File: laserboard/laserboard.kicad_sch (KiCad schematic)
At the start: 32 parts, among them U1 AD8656 (1/2 equivalent), U2 AD8656 (1/2 equivalent), U3 AD8656 (1/2 equivalent), U4 AD8656 (1/2 equivalent)

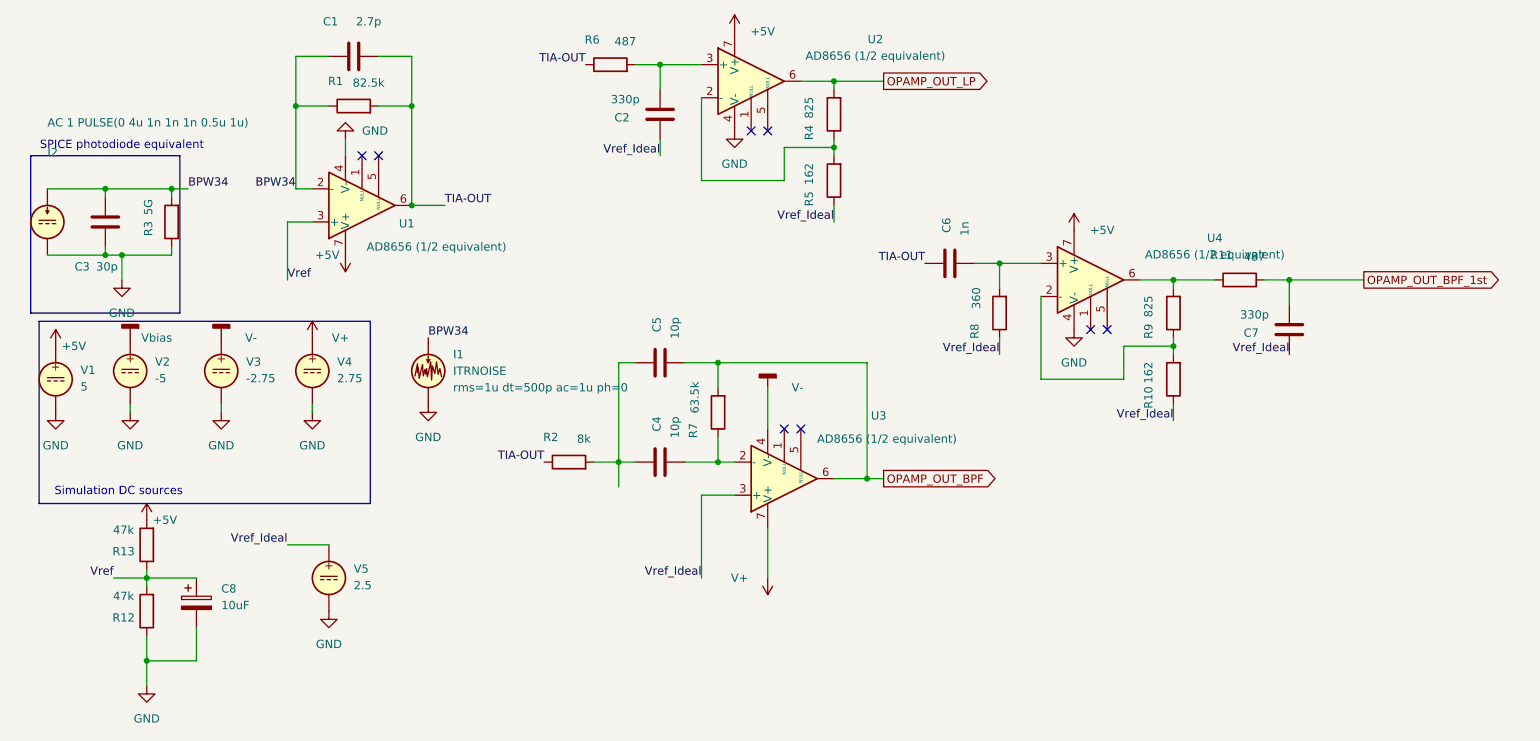
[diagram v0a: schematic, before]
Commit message: Backup
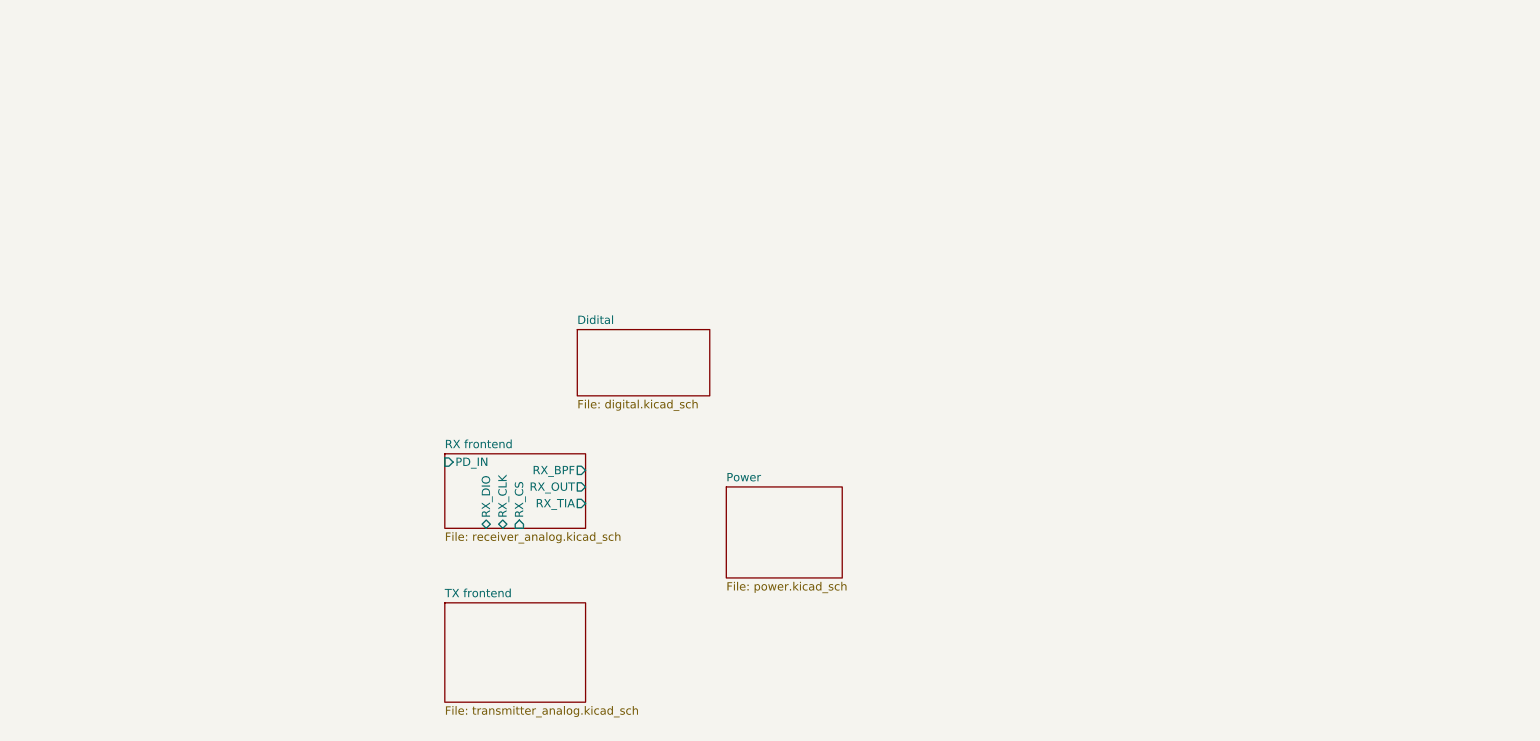
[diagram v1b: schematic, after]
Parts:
- removed C1: 2.7p, symbol Device:C
- removed C2, C7: 330p, symbol Device:C
- removed C3: 30p, symbol Device:C
- removed C4, C5: 10p, symbol Device:C
- removed C6: 1n, symbol Device:C
- removed C8: 10uF, symbol Device:C_Polarized
- removed I1: ITRNOISE, symbol Simulation_SPICE:ITRNOISE
- removed I2: AC 1 PULSE(0 4u 1n 1n 1n 0.5u 1u), symbol Simulation_SPICE:IDC
- removed R1: 82.5k, symbol Device:R
- removed R10, R5: 162, symbol Device:R
- removed R11, R6: 487, symbol Device:R
- removed R12, R13: 47k, symbol Device:R
- removed R2: 8k, symbol Device:R
- removed R3: 5G, symbol Device:R
- removed R4, R9: 825, symbol Device:R
- removed R7: 63.5k, symbol Device:R
- removed R8: 360, symbol Device:R
- removed U1, U2, U3, U4: AD8656 (1/2 equivalent), symbol Amplifier_Operational:AD8655
- removed V1: 5, symbol Simulation_SPICE:VDC
- removed V2: -5, symbol Simulation_SPICE:VDC
- removed V3: -2.75, symbol Simulation_SPICE:VDC
- removed V4: 2.75, symbol Simulation_SPICE:VDC
- removed V5: 2.5, symbol Simulation_SPICE:VDC
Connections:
- no-connect marks 8 -> 0
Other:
- added sheet Didital (digital.kicad_sch)
- added sheet Power (power.kicad_sch)
- added sheet RX frontend (receiver_analog.kicad_sch)
- added sheet TX frontend (transmitter_analog.kicad_sch)
- note removed: "SPICE photodiode equivalent"
- note removed: "Simulation DC sources"
